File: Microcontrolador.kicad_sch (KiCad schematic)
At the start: 1 part, among them IC2 R7F125FPL4AFB-C#UA0

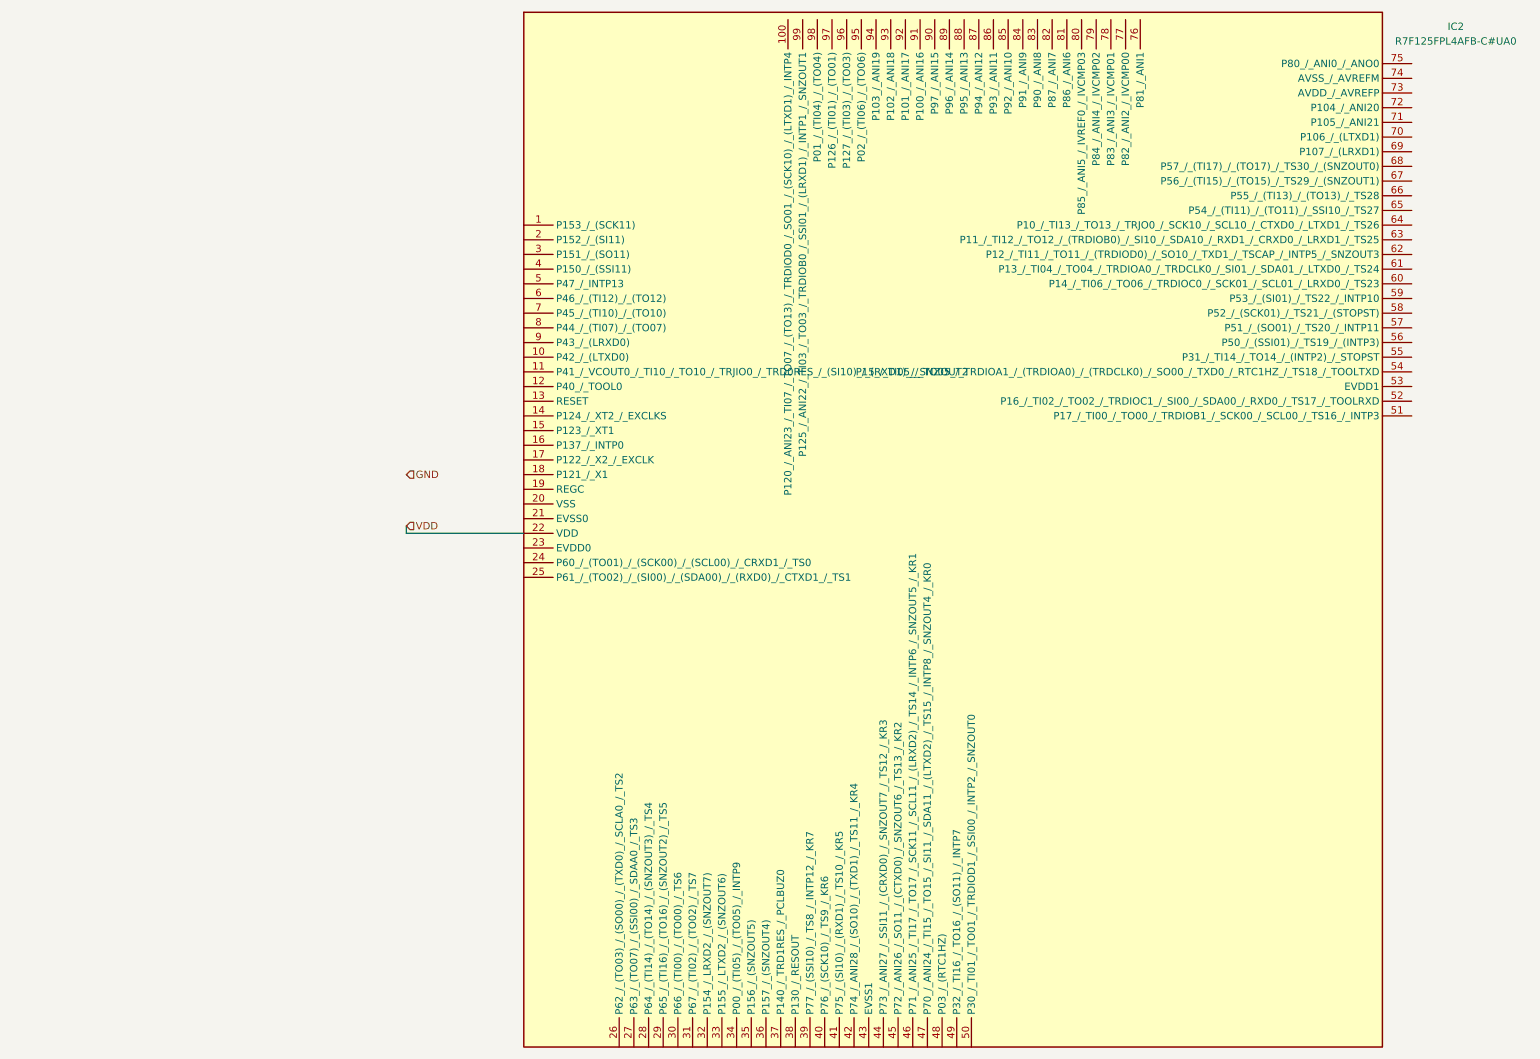
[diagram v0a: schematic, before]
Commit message: He corregido los errores de la tarea 2 y he añadido los condensadores de desacople.
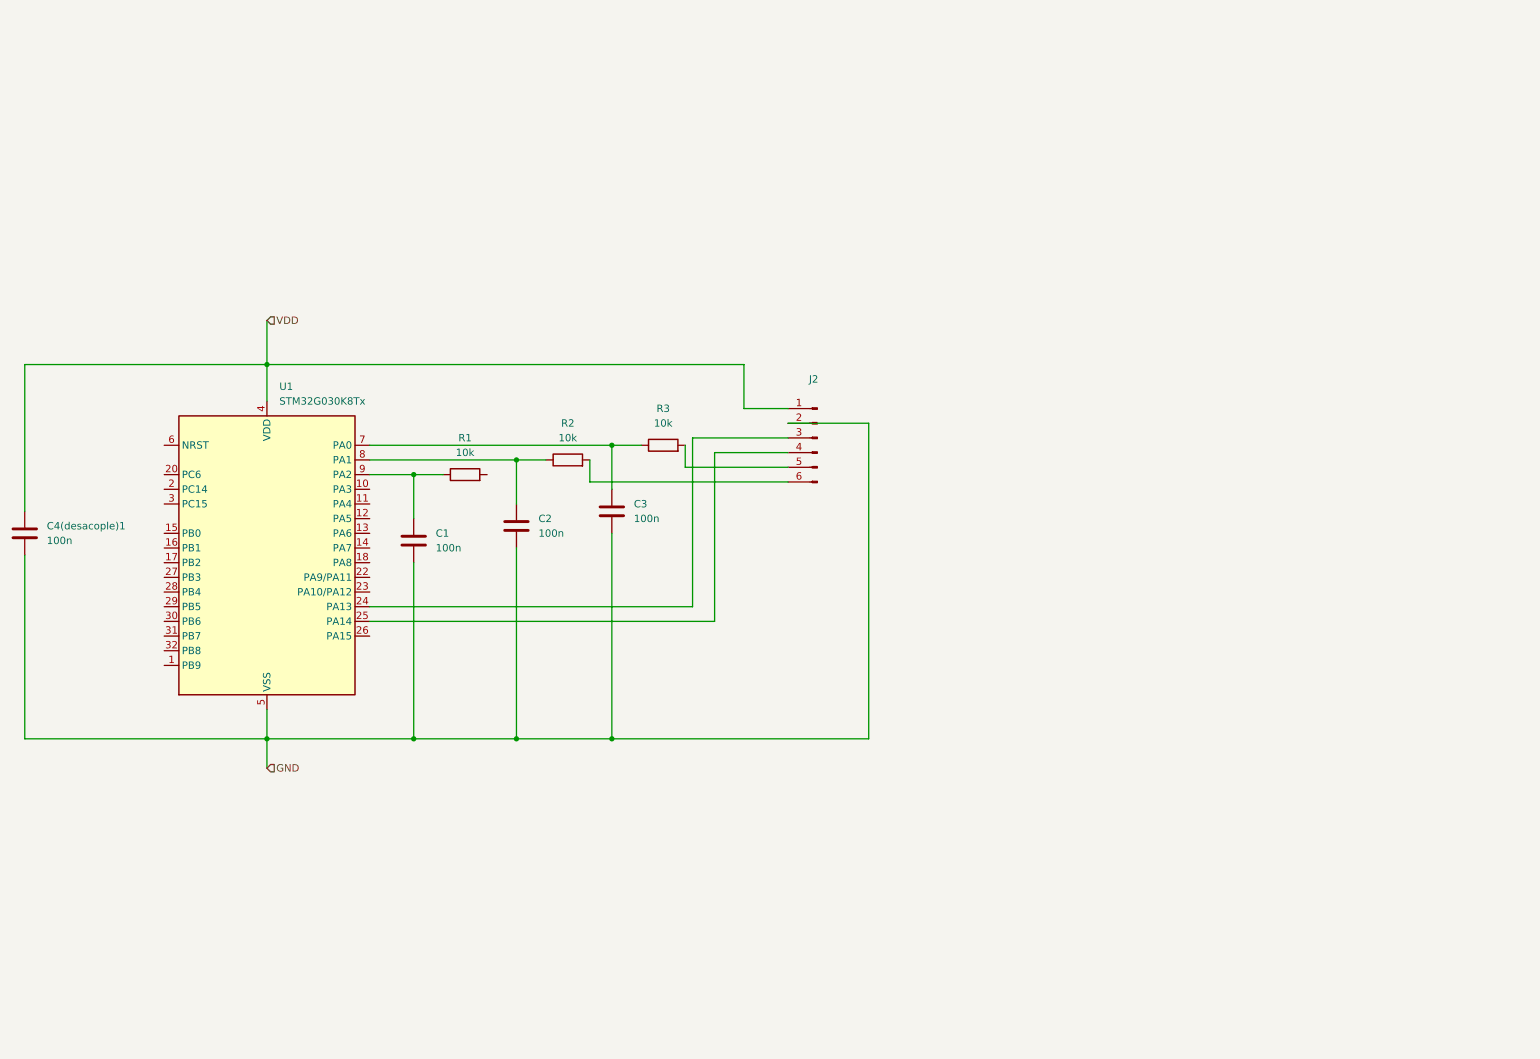
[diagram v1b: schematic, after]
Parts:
- removed IC2: R7F125FPL4AFB-C#UA0, QFP50P1600X1600X160-100N, symbol R7F125FPL4AFB-C#UA0:R7F125FPL4AFB-C#UA0
- added C1, C2, C3, C4(desacople)1: 100n, Capacitor_SMD:C_0805_2012Metric, symbol Device:C
- added J2: Conn_01x06_Pin, Connector_PinHeader_2.54mm:PinHeader_1x06_P2.54mm_Horizontal, symbol Connector:Conn_01x06_Pin
- added R1, R2, R3: 10k, Resistor_SMD:R_0805_2012Metric, symbol Device:R
- added U1: STM32G030K8Tx, Package_QFP:LQFP-32_7x7mm_P0.8mm, symbol MCU_ST_STM32G0:STM32G030K8Tx
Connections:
- net GND: now also C1.2, C2.2, C3.2, C4(desacople)1.2, J2.2 (Pin_2), U1.5 (VSS)
- net VDD: now also C4(desacople)1.1, J2.1 (Pin_1), U1.4 (VDD)
- new net: C3.1, R3.1, U1.7 (PA0)
- new net: C2.1, R2.1, U1.8 (PA1)
- new net: J2.6 (Pin_6), R2.2
- new net: C1.1, R1.1, U1.9 (PA2)
- new net: J2.5 (Pin_5), R3.2
- new net: J2.3 (Pin_3), U1.24 (PA13)
- new net: J2.4 (Pin_4), U1.25 (PA14)
